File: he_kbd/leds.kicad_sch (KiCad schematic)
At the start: 73 parts

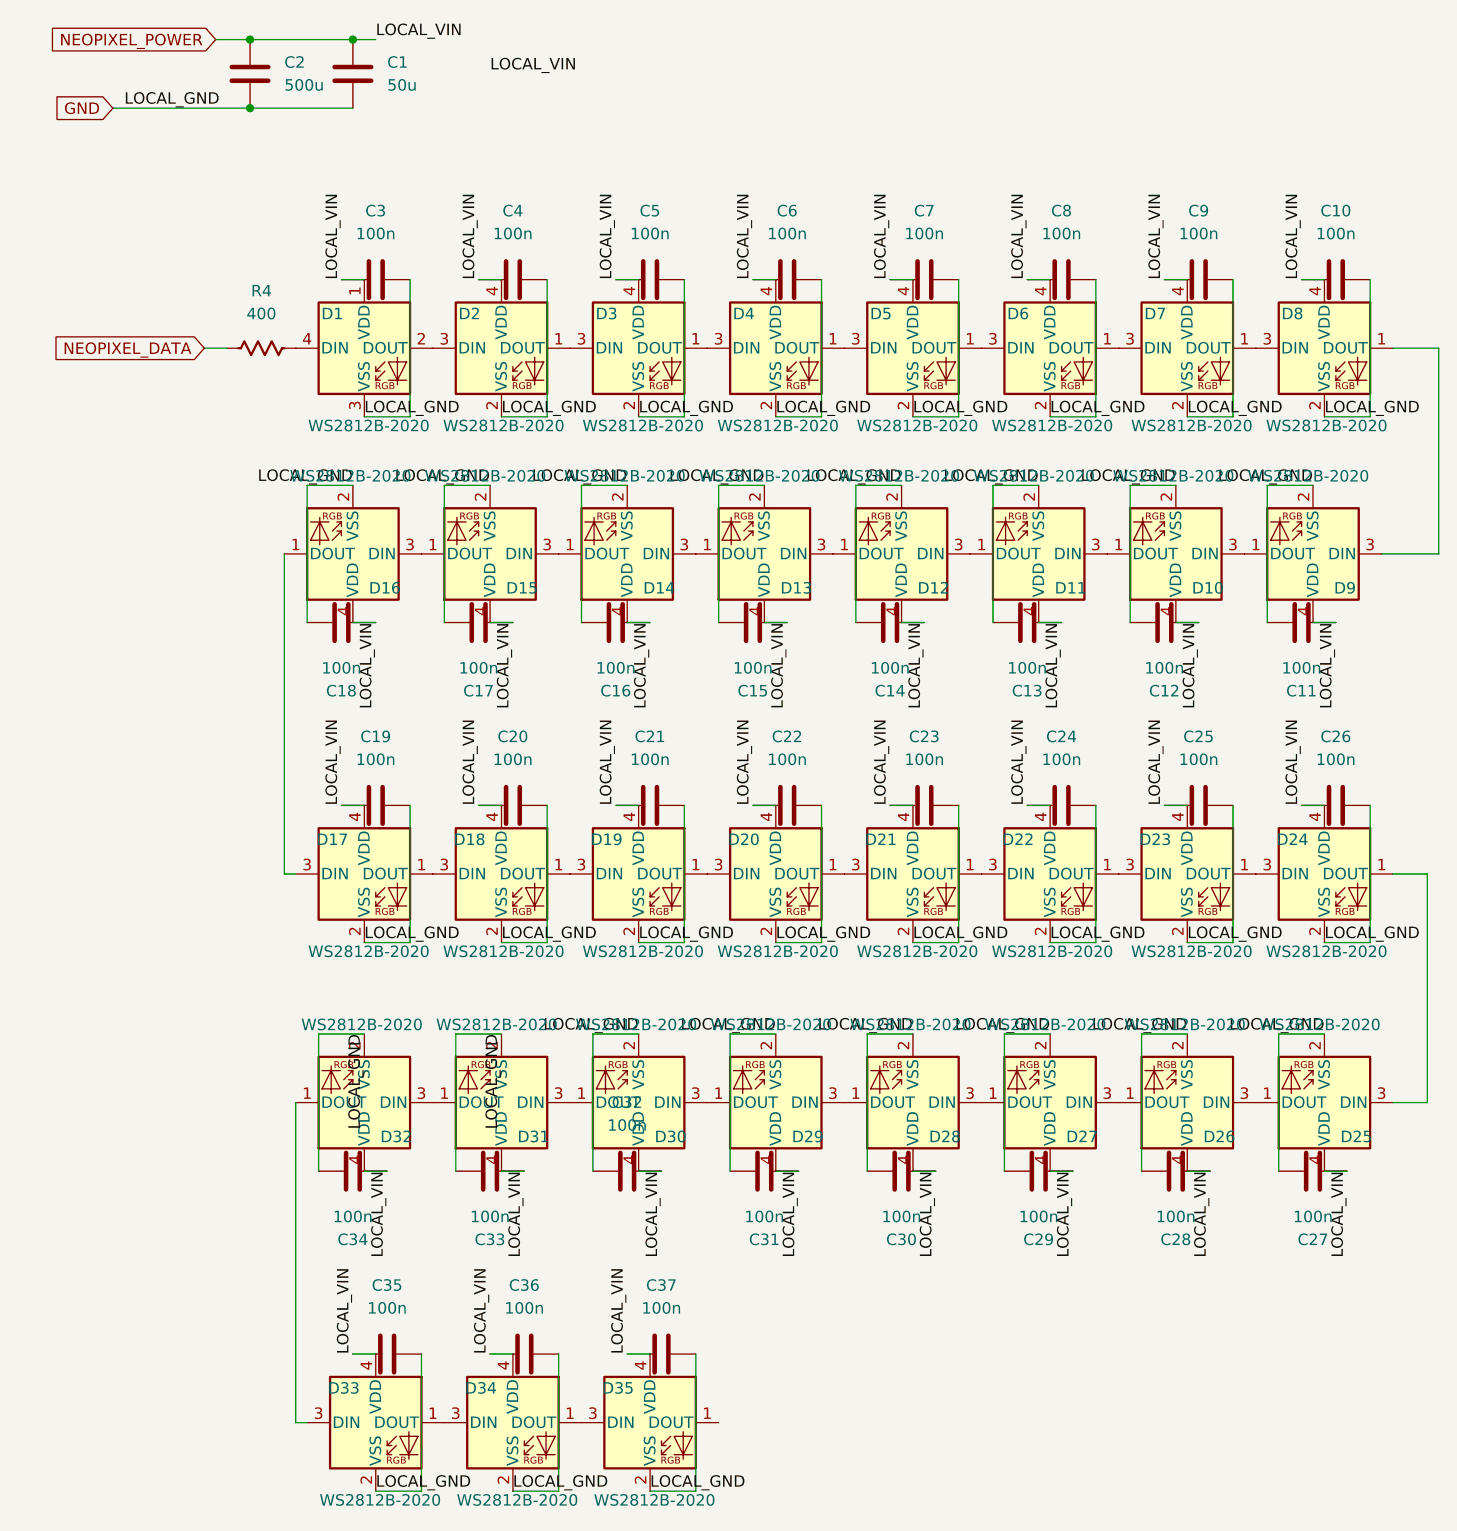
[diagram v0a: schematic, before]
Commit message: now have to fix all footprints for the leds and decoupling capacitors
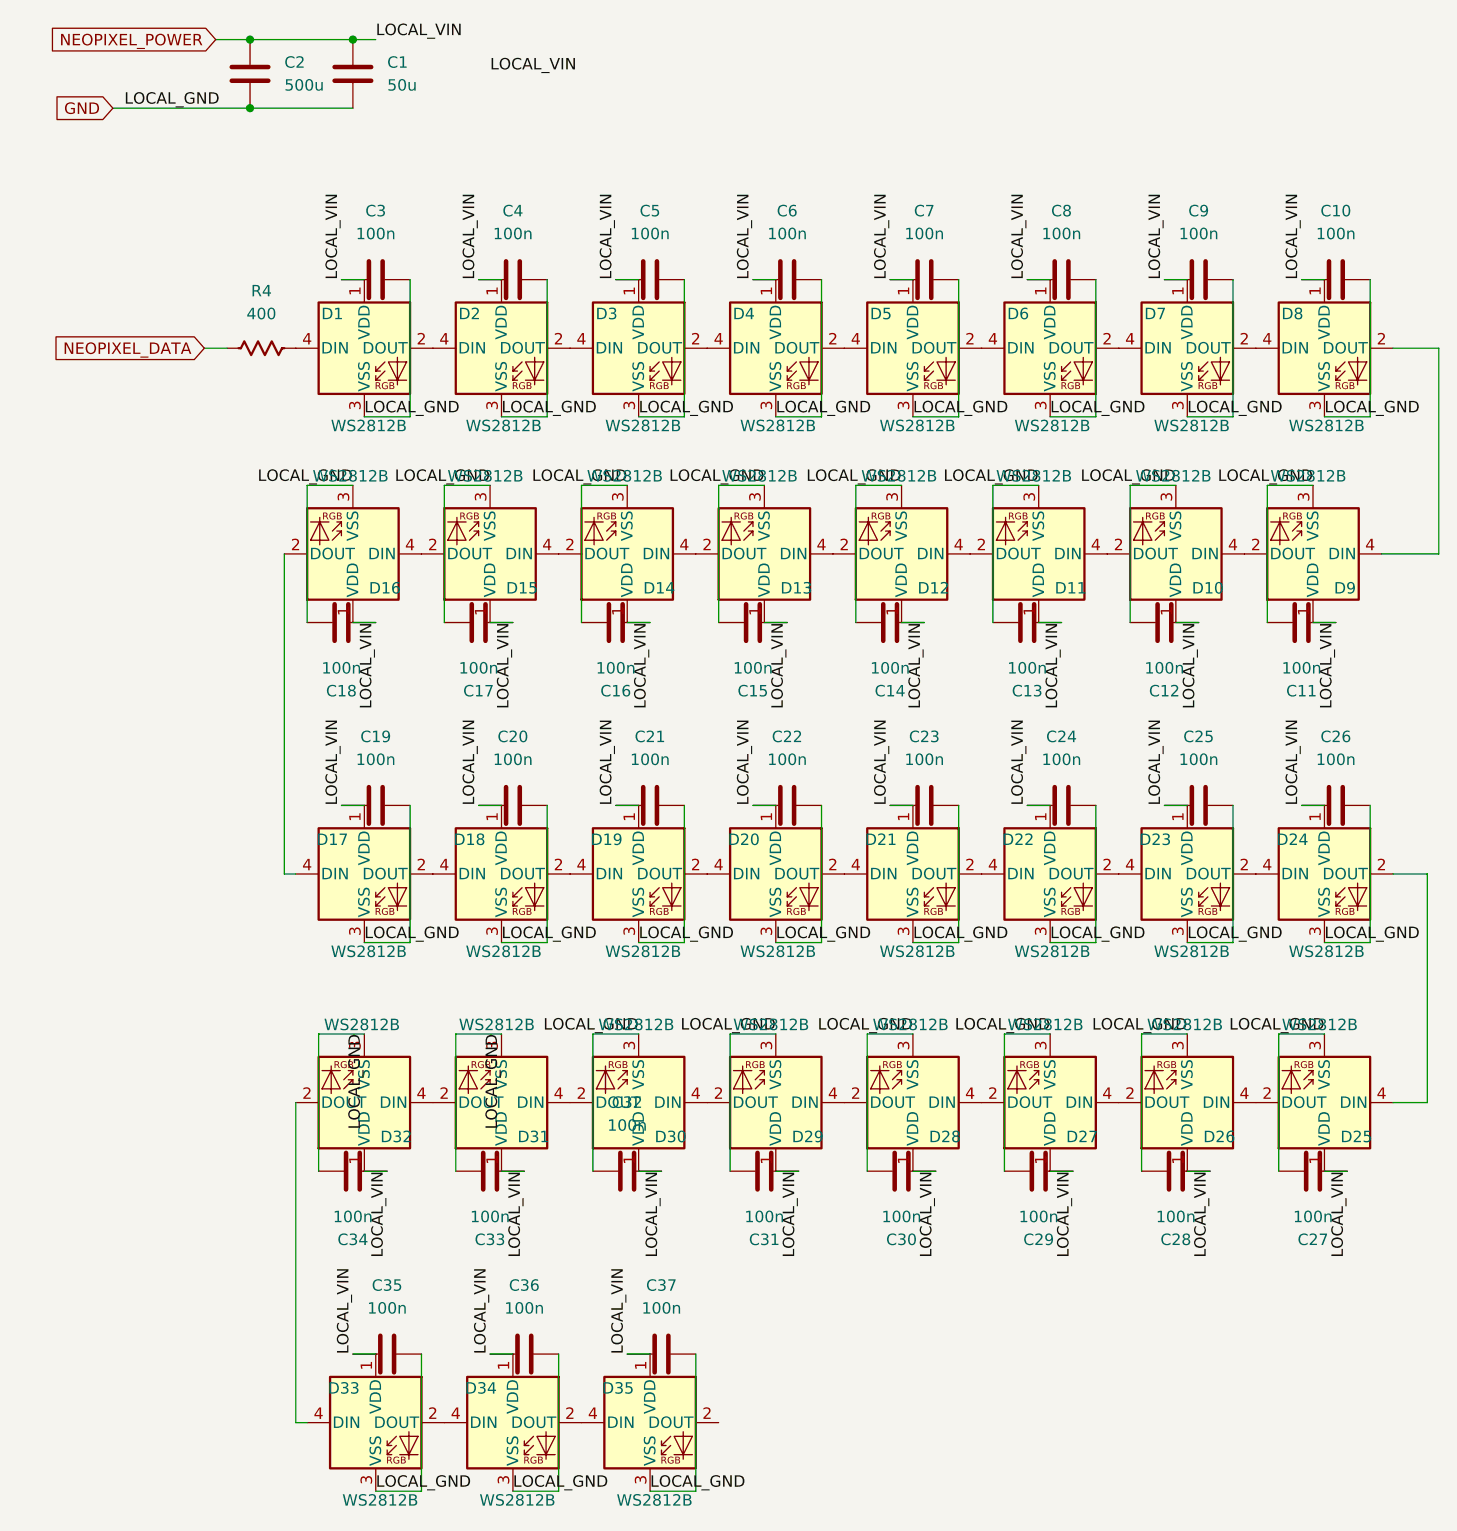
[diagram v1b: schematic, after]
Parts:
- D1: value WS2812B-2020 -> WS2812B
- D10, D11, D12, D13, D14, D15, D16, D17, D18, D19, D2, D20, D21, D22, D23, D24, D25, D26, D27, D28, D29, D3, D30, D31, D32, D33, D34, D35, D4, D5, D6, D7, D8, D9: value WS2812B-2020 -> WS2812B; footprint LED_SMD:LED_WS2812B-2020_PLCC4_2.0x2.0mm -> LED_SMD:LED_WS2812B_PLCC4_5.0x5.0mm_P3.2mm; symbol LED:WS2812B-2020 -> LED:WS2812B
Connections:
- net GND: now also D10.3 (VSS), D11.3 (VSS), D12.3 (VSS), D13.3 (VSS), D14.3 (VSS), D15.3 (VSS), D16.3 (VSS), D17.3 (VSS), D18.3 (VSS), D19.3 (VSS), D2.3 (VSS), D20.3 (VSS), D21.3 (VSS), D22.3 (VSS), D23.3 (VSS), D24.3 (VSS), D25.3 (VSS), D26.3 (VSS), D27.3 (VSS), D28.3 (VSS), D29.3 (VSS), D3.3 (VSS), D30.3 (VSS), D31.3 (VSS), D32.3 (VSS), D33.3 (VSS), D34.3 (VSS), D35.3 (VSS), D4.3 (VSS), D5.3 (VSS), D6.3 (VSS), D7.3 (VSS), D8.3 (VSS), D9.3 (VSS); no longer D10.2 (VSS), D11.2 (VSS), D12.2 (VSS), D13.2 (VSS), D14.2 (VSS), D15.2 (VSS), D16.2 (VSS), D17.2 (VSS), D18.2 (VSS), D19.2 (VSS), D2.2 (VSS), D20.2 (VSS), D21.2 (VSS), D22.2 (VSS), D23.2 (VSS), D24.2 (VSS), D25.2 (VSS), D26.2 (VSS), D27.2 (VSS), D28.2 (VSS), D29.2 (VSS), D3.2 (VSS), D30.2 (VSS), D31.2 (VSS), D32.2 (VSS), D33.2 (VSS), D34.2 (VSS), D35.2 (VSS), D4.2 (VSS), D5.2 (VSS), D6.2 (VSS), D7.2 (VSS), D8.2 (VSS), D9.2 (VSS)
- net NEOPIXEL_POWER: now also D10.1 (VDD), D11.1 (VDD), D12.1 (VDD), D13.1 (VDD), D14.1 (VDD), D15.1 (VDD), D16.1 (VDD), D17.1 (VDD), D18.1 (VDD), D19.1 (VDD), D2.1 (VDD), D20.1 (VDD), D21.1 (VDD), D22.1 (VDD), D23.1 (VDD), D24.1 (VDD), D25.1 (VDD), D26.1 (VDD), D27.1 (VDD), D28.1 (VDD), D29.1 (VDD), D3.1 (VDD), D30.1 (VDD), D31.1 (VDD), D32.1 (VDD), D33.1 (VDD), D34.1 (VDD), D35.1 (VDD), D4.1 (VDD), D5.1 (VDD), D6.1 (VDD), D7.1 (VDD), D8.1 (VDD), D9.1 (VDD); no longer D10.4 (VDD), D11.4 (VDD), D12.4 (VDD), D13.4 (VDD), D14.4 (VDD), D15.4 (VDD), D16.4 (VDD), D17.4 (VDD), D18.4 (VDD), D19.4 (VDD), D2.4 (VDD), D20.4 (VDD), D21.4 (VDD), D22.4 (VDD), D23.4 (VDD), D24.4 (VDD), D25.4 (VDD), D26.4 (VDD), D27.4 (VDD), D28.4 (VDD), D29.4 (VDD), D3.4 (VDD), D30.4 (VDD), D31.4 (VDD), D32.4 (VDD), D33.4 (VDD), D34.4 (VDD), D35.4 (VDD), D4.4 (VDD), D5.4 (VDD), D6.4 (VDD), D7.4 (VDD), D8.4 (VDD), D9.4 (VDD)
- net at D1.2 (DOUT): now also D2.4 (DIN); no longer D2.3 (DIN)
- new net: D12.2 (DOUT), D13.4 (DIN)
- new net: D11.2 (DOUT), D12.4 (DIN)
- new net: D16.2 (DOUT), D17.4 (DIN)
- new net: D15.2 (DOUT), D16.4 (DIN)
- new net: D8.2 (DOUT), D9.4 (DIN)
- new net: D7.2 (DOUT), D8.4 (DIN)
- new net: D22.2 (DOUT), D23.4 (DIN)
- new net: D21.2 (DOUT), D22.4 (DIN)
- new net: D13.2 (DOUT), D14.4 (DIN)
- new net: D18.2 (DOUT), D19.4 (DIN)
- new net: D17.2 (DOUT), D18.4 (DIN)
- new net: D6.2 (DOUT), D7.4 (DIN)
- new net: D5.2 (DOUT), D6.4 (DIN)
- new net: D4.2 (DOUT), D5.4 (DIN)
- new net: D25.2 (DOUT), D26.4 (DIN)
- new net: D24.2 (DOUT), D25.4 (DIN)
- new net: D27.2 (DOUT), D28.4 (DIN)
- new net: D26.2 (DOUT), D27.4 (DIN)
- new net: D3.2 (DOUT), D4.4 (DIN)
- new net: D14.2 (DOUT), D15.4 (DIN)
- new net: D34.2 (DOUT), D35.4 (DIN)
- new net: D33.2 (DOUT), D34.4 (DIN)
- new net: D19.2 (DOUT), D20.4 (DIN)
- new net: D10.4 (DIN), D9.2 (DOUT)
- new net: D23.2 (DOUT), D24.4 (DIN)
- new net: D32.2 (DOUT), D33.4 (DIN)
- new net: D10.2 (DOUT), D11.4 (DIN)
- new net: D30.2 (DOUT), D31.4 (DIN)
- new net: D29.2 (DOUT), D30.4 (DIN)
- new net: D28.2 (DOUT), D29.4 (DIN)
- new net: D31.2 (DOUT), D32.4 (DIN)
- new net: D20.2 (DOUT), D21.4 (DIN)
- new net: D2.2 (DOUT), D3.4 (DIN)
